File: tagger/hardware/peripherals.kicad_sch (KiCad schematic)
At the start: 15 parts, among them J2 MICRO_SD_CARD, U1 LSM6DS3, U8 MAX98357A, U9 W25Q128JVP

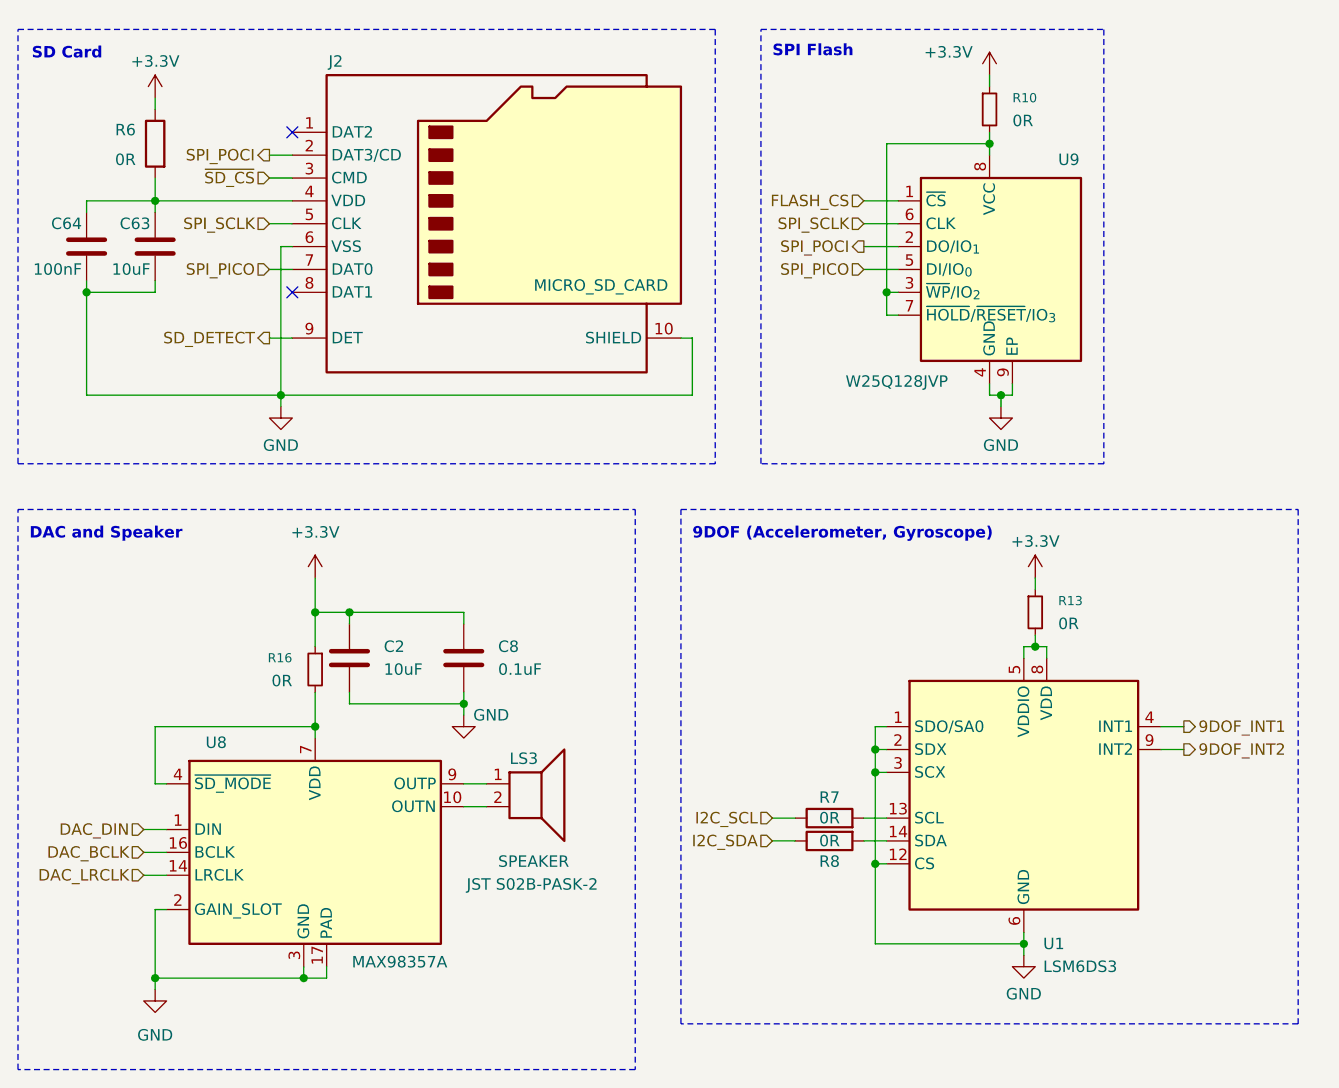
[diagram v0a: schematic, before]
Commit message: feat: added missing 3d models
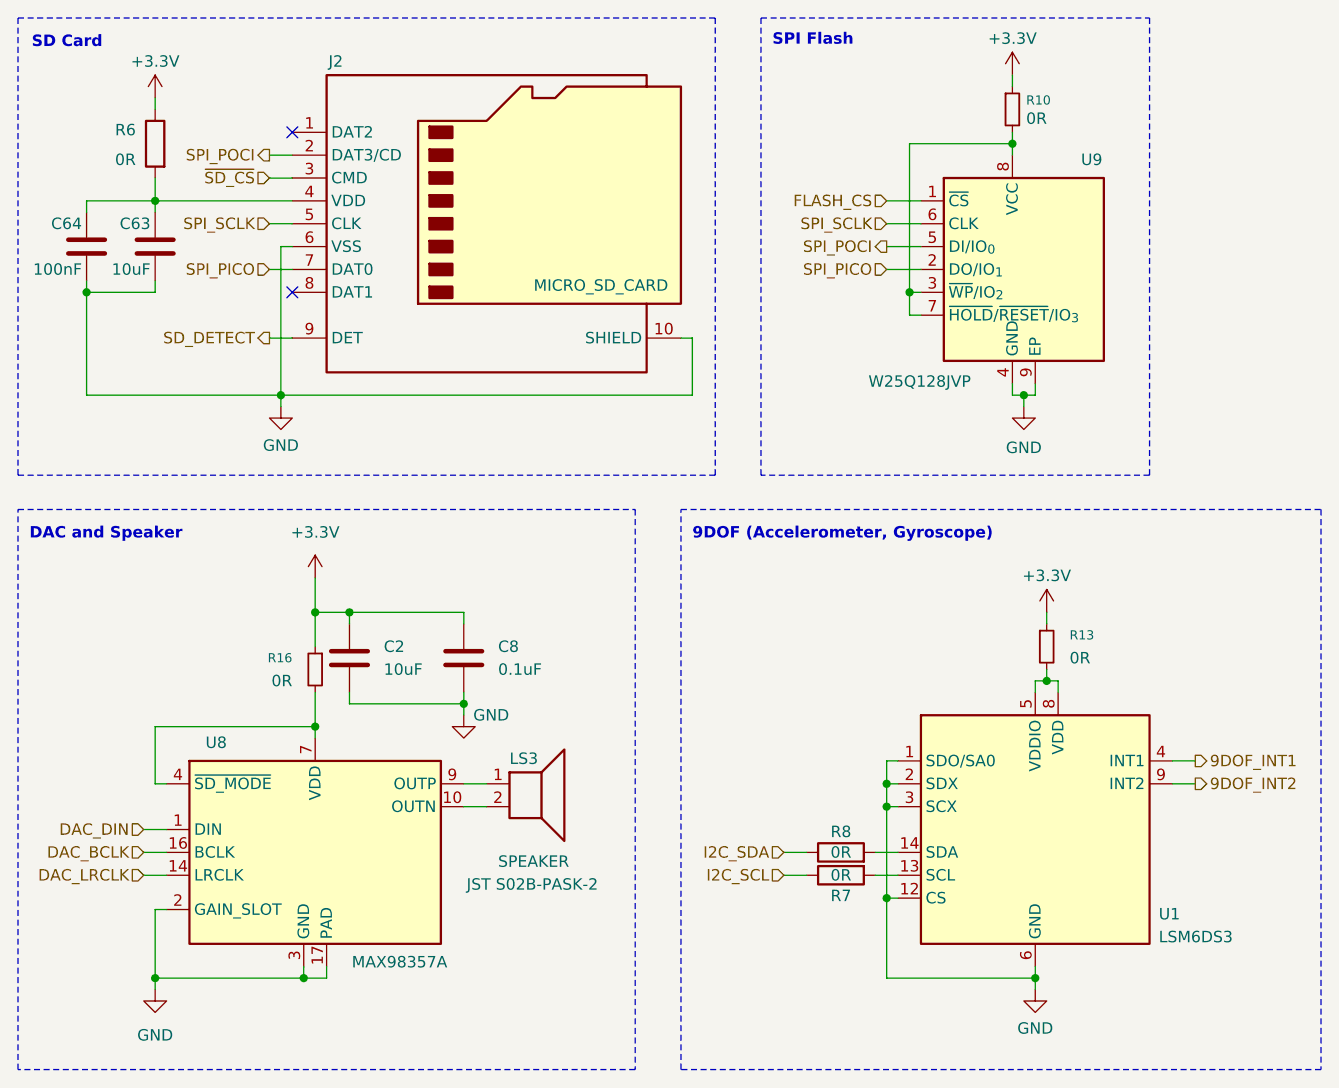
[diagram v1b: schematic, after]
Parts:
- LS3: footprint Connector_PinHeader_2.00mm:PinHeader_1x02_P2.00mm_Horizontal -> tagger:S02B-PASK-2
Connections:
- net SPI_PICO: now also U9.2 (DO/IO_{1}); no longer U9.5 (DI/IO_{0})
- net SPI_POCI: now also U9.5 (DI/IO_{0}); no longer U9.2 (DO/IO_{1})
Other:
- moved on the sheet: R10, R13, R7, R8, U1, U9
